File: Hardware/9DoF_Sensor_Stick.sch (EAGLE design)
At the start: 31 parts, among them U1 ITG-3200, U2 ADXL345, U4 3.3V

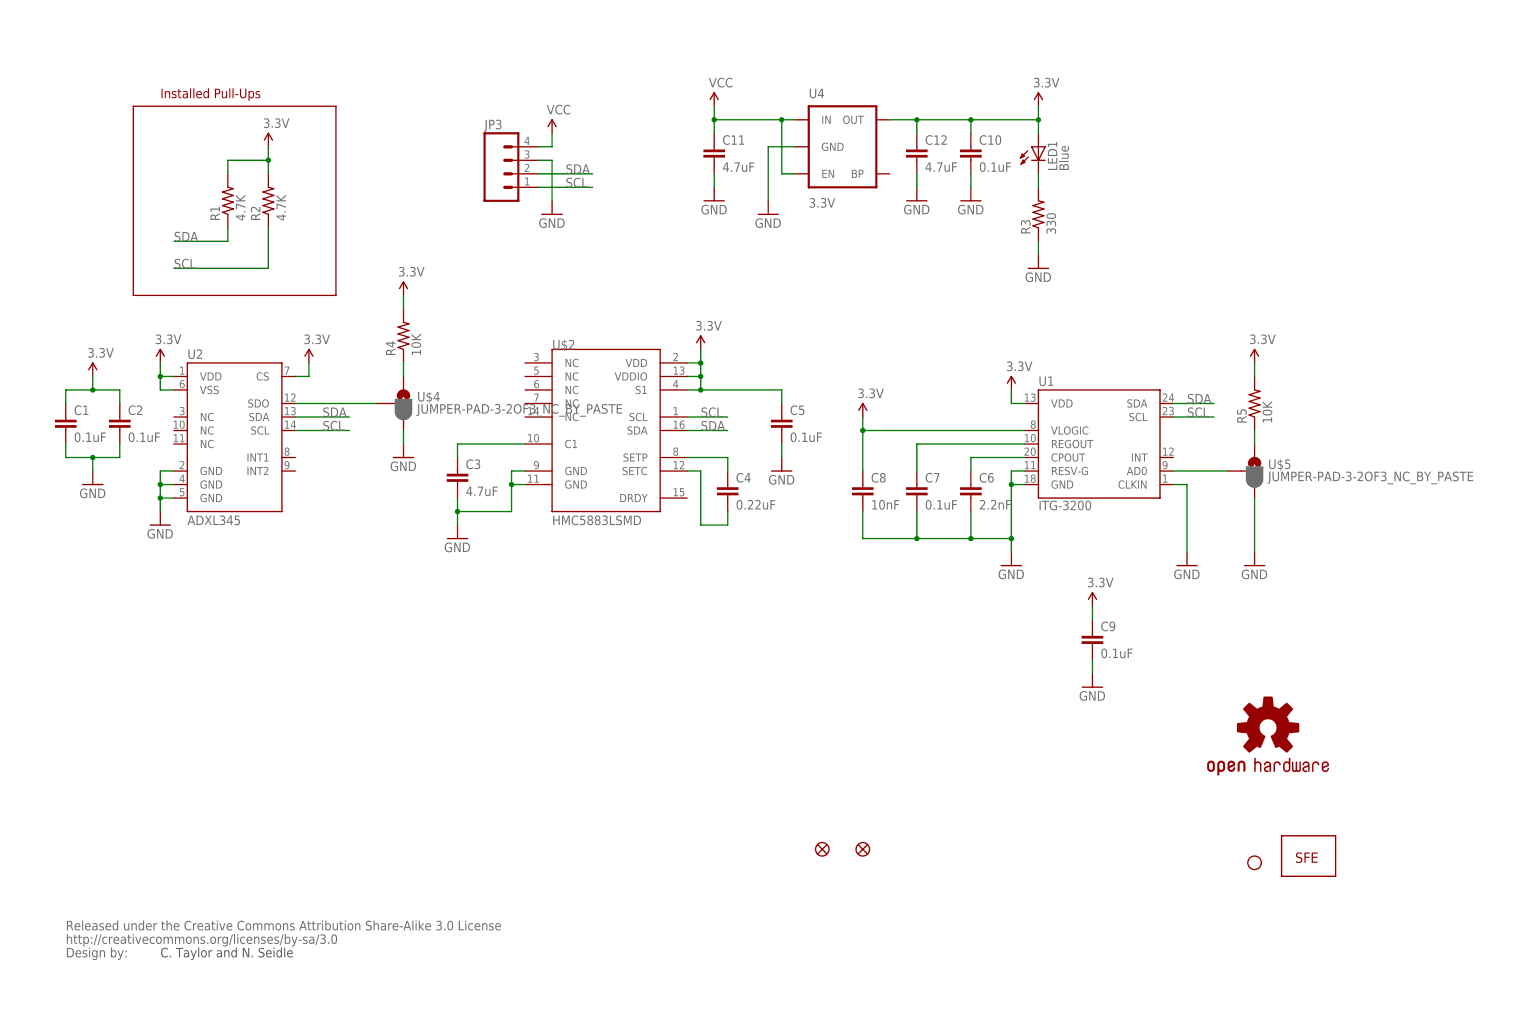
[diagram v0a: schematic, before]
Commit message: comp change
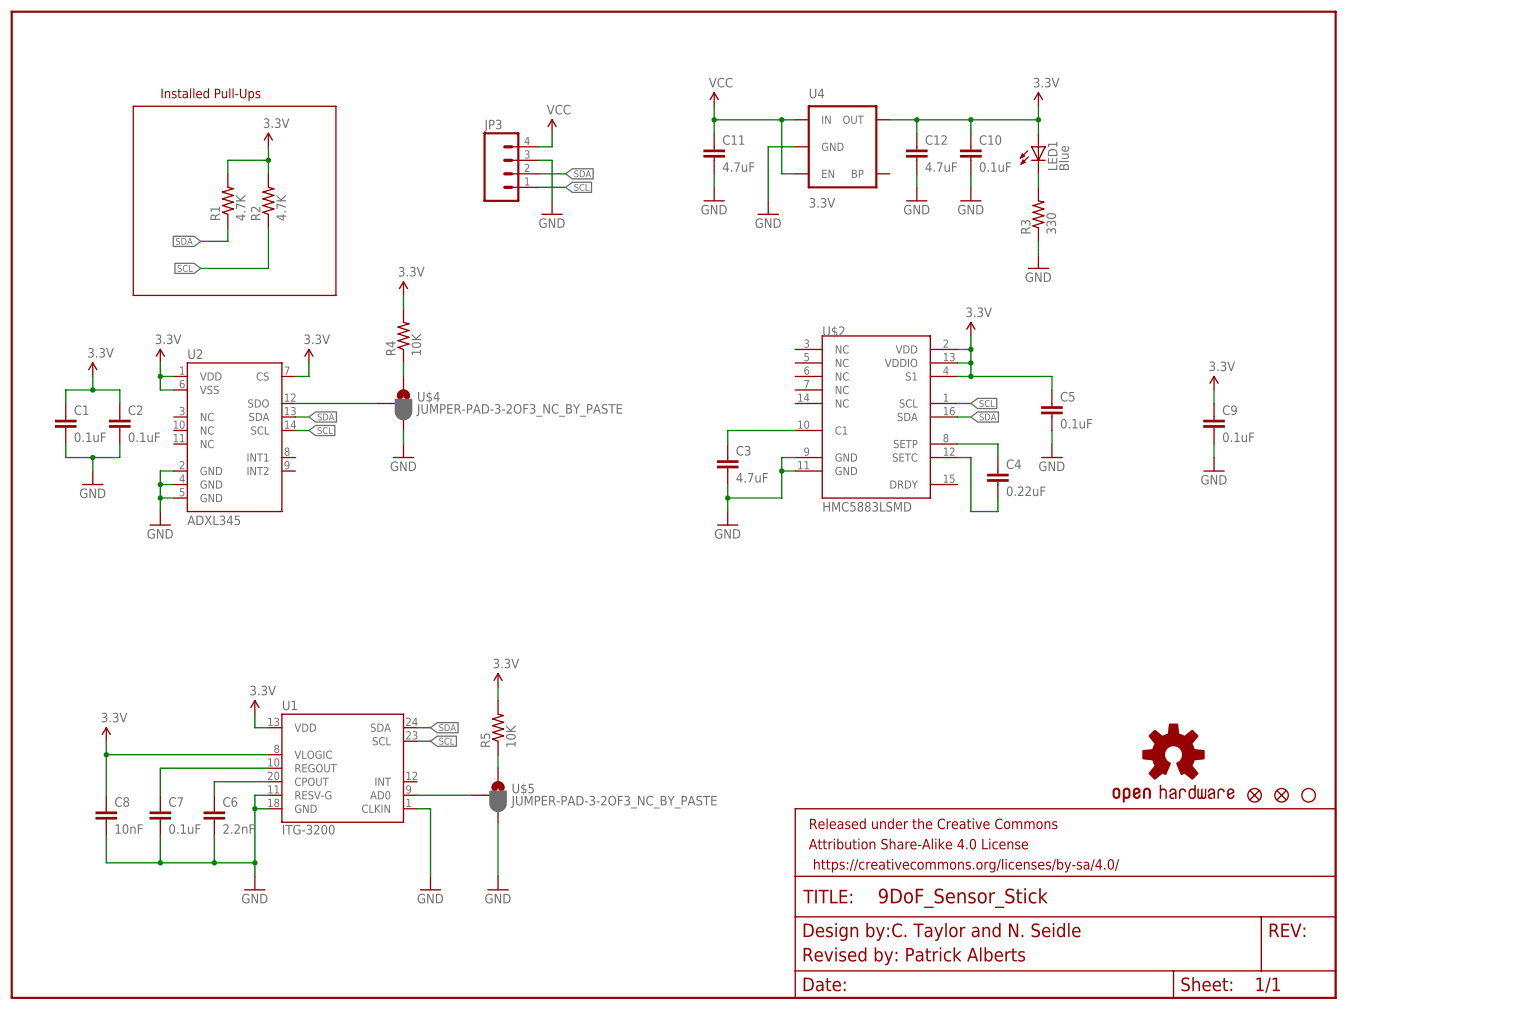
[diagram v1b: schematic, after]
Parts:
- removed JP4: LOGO-SFESK, SparkFun:LOGO-SFESK
- removed U$1: CREATIVE_COMMONS, SparkFun:CREATIVE_COMMONS
- added FRAME1: FRAME-LETTER, SparkFun-Aesthetics:FRAME-LETTER
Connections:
- net N$10: now also U$5.2
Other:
- note added: "Revised by: Patrick Alberts"
- moved on the sheet: C3, C4, C5, C6, C7, C8, C9, R5, U$2, U$5, U1
